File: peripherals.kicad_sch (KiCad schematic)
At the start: 64 parts, among them SW1 USER, SW2 BOOTSEL, SW3 RESET, U2 ATECC608A-MAHDA, U3 W25Q128XXX

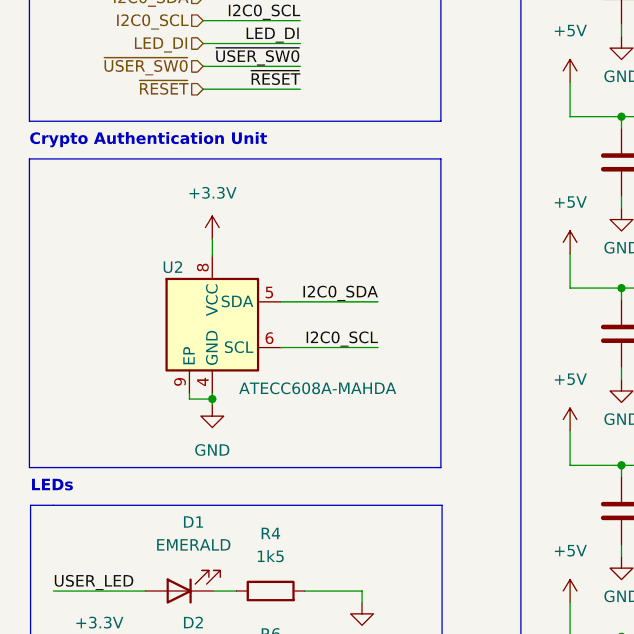
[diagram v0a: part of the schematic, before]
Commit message: Production Design V1.0
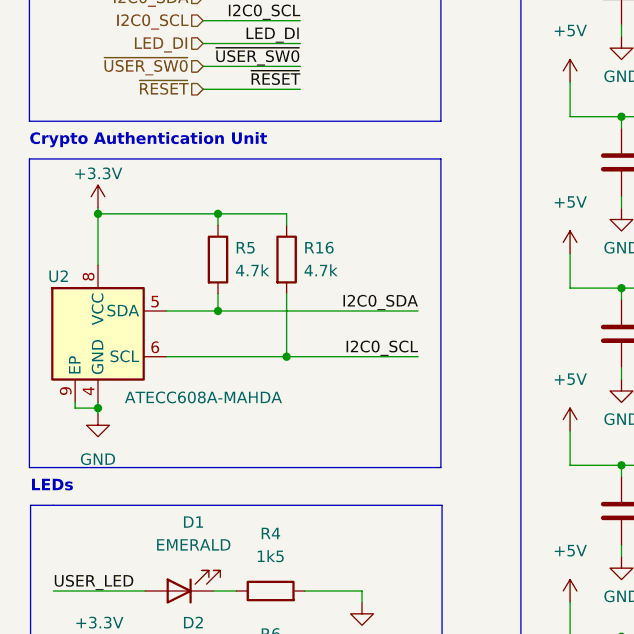
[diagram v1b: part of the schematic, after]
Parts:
- added R16, R5: 4.7k, Resistor_SMD:R_0402_1005Metric, symbol Device:R
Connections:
- net +3V3: now also R16.1, R5.1
- net I2C0_SCL: now also R16.2
- net I2C0_SDA: now also R5.2
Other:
- moved on the sheet: U2
